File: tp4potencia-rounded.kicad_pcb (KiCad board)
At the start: 2 copper layers, 130 x 115 mm, 88 parts, among them J2 Screw_Terminal_01x03, J3 Screw_Terminal_01x02, Q1 IRF840, Q2 IRF840, SW2 SW_SPDT, SW4 SW_SPDT, T1 Trafo1, U1 LTV-817, U2 IR2110, U3 SG3525, U4 LM339

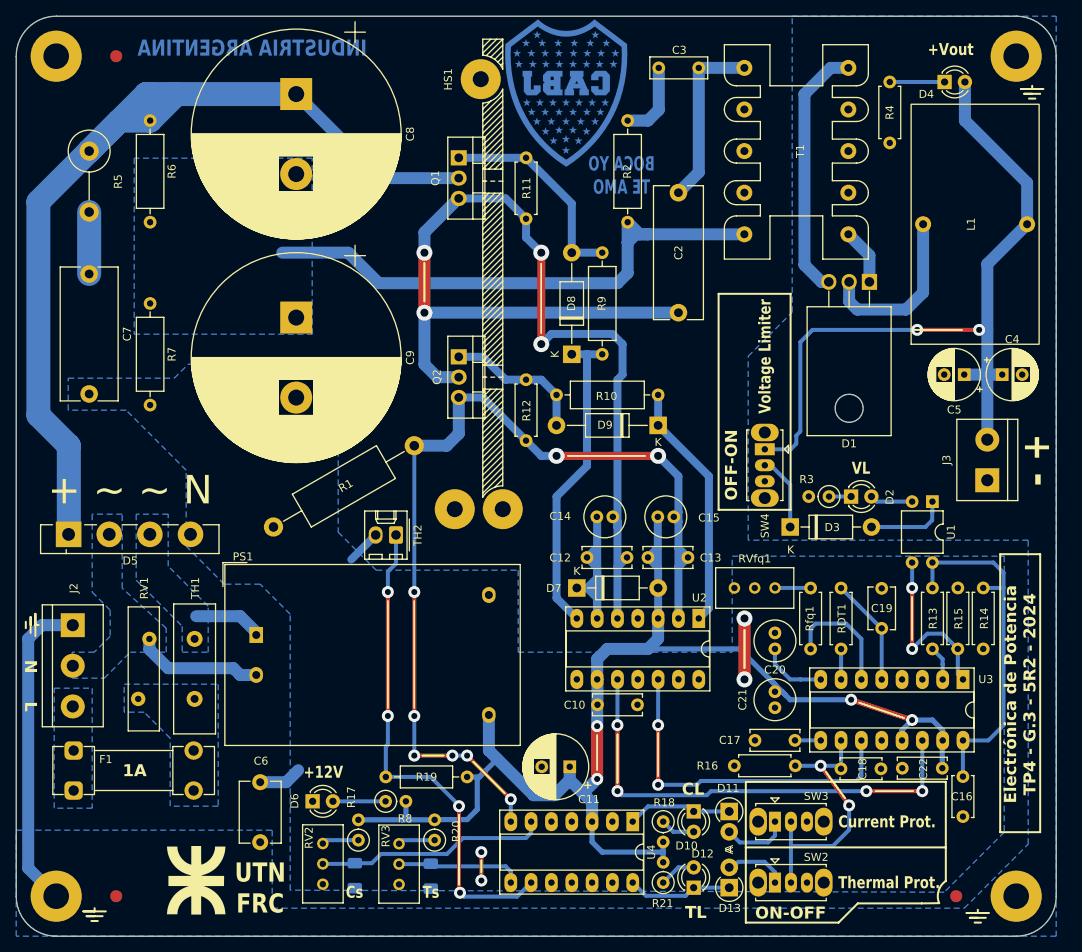
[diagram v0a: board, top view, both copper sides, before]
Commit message: Ver 1.0
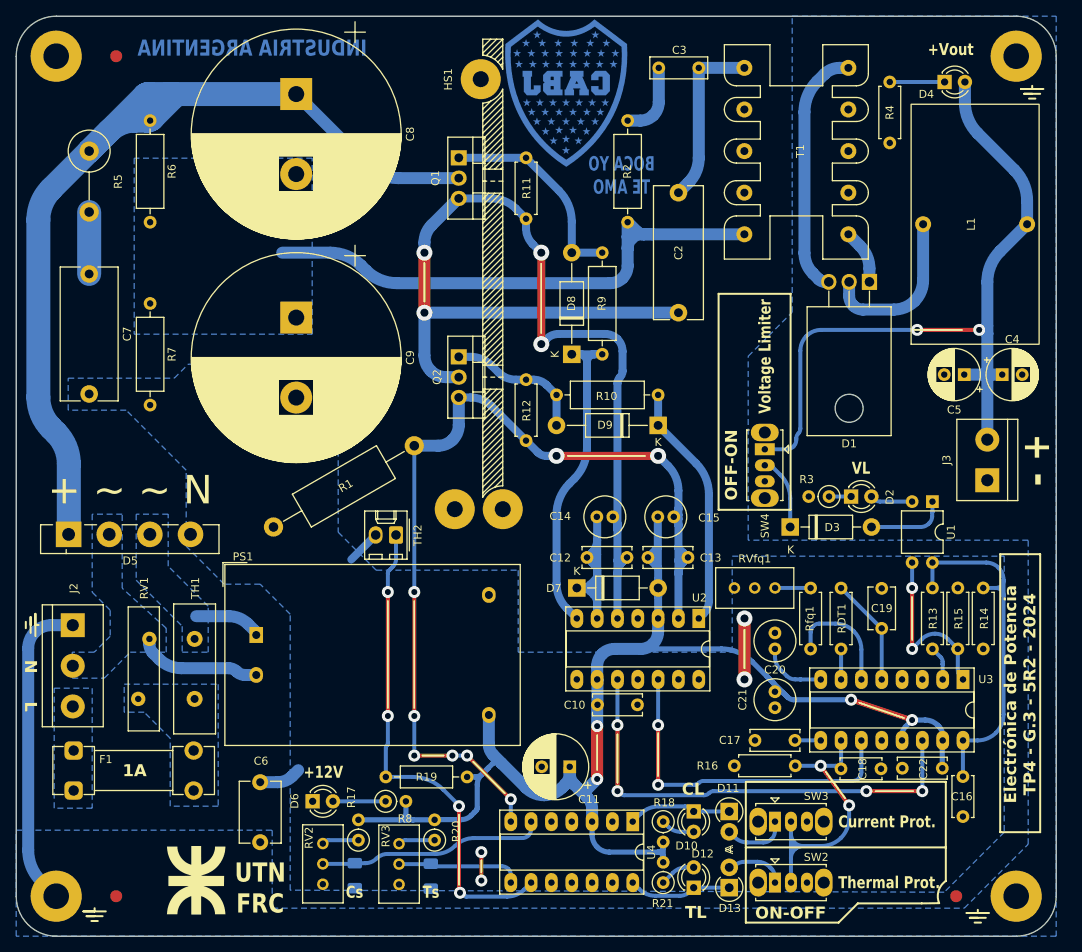
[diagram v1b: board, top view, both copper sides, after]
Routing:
- net +12V: track 167.2 -> 177.2 mm
- net Net-(D7-K): track 29.4 -> 34.3 mm
- net /PWM/SHUTDOWN: track 34.3 -> 37.9 mm
- net /Sl: track 121.1 -> 123.0 mm
- net /PWM/VREF: track 44.6 -> 46.0 mm
- net Net-(D8-K): track 39.5 -> 40.7 mm
- net +155V: track 69.8 -> 70.8 mm
- net +310V: track 124.3 -> 123.5 mm
- net /Sh: track 134.1 -> 134.8 mm
- net Net-(U4B--): track 29.0 -> 28.4 mm
- net /T1: track 32.1 -> 31.5 mm
- net Net-(U4D-+): track 62.2 -> 61.6 mm
- net GND: track 39.9 -> 39.4 mm
- net /T0: track 21.5 -> 21.0 mm
